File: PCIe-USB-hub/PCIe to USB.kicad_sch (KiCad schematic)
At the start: 105 parts, among them Y1 X322524MQB4SI, Y2 X322524MQB4SI, Y3 X322524MQB4SI

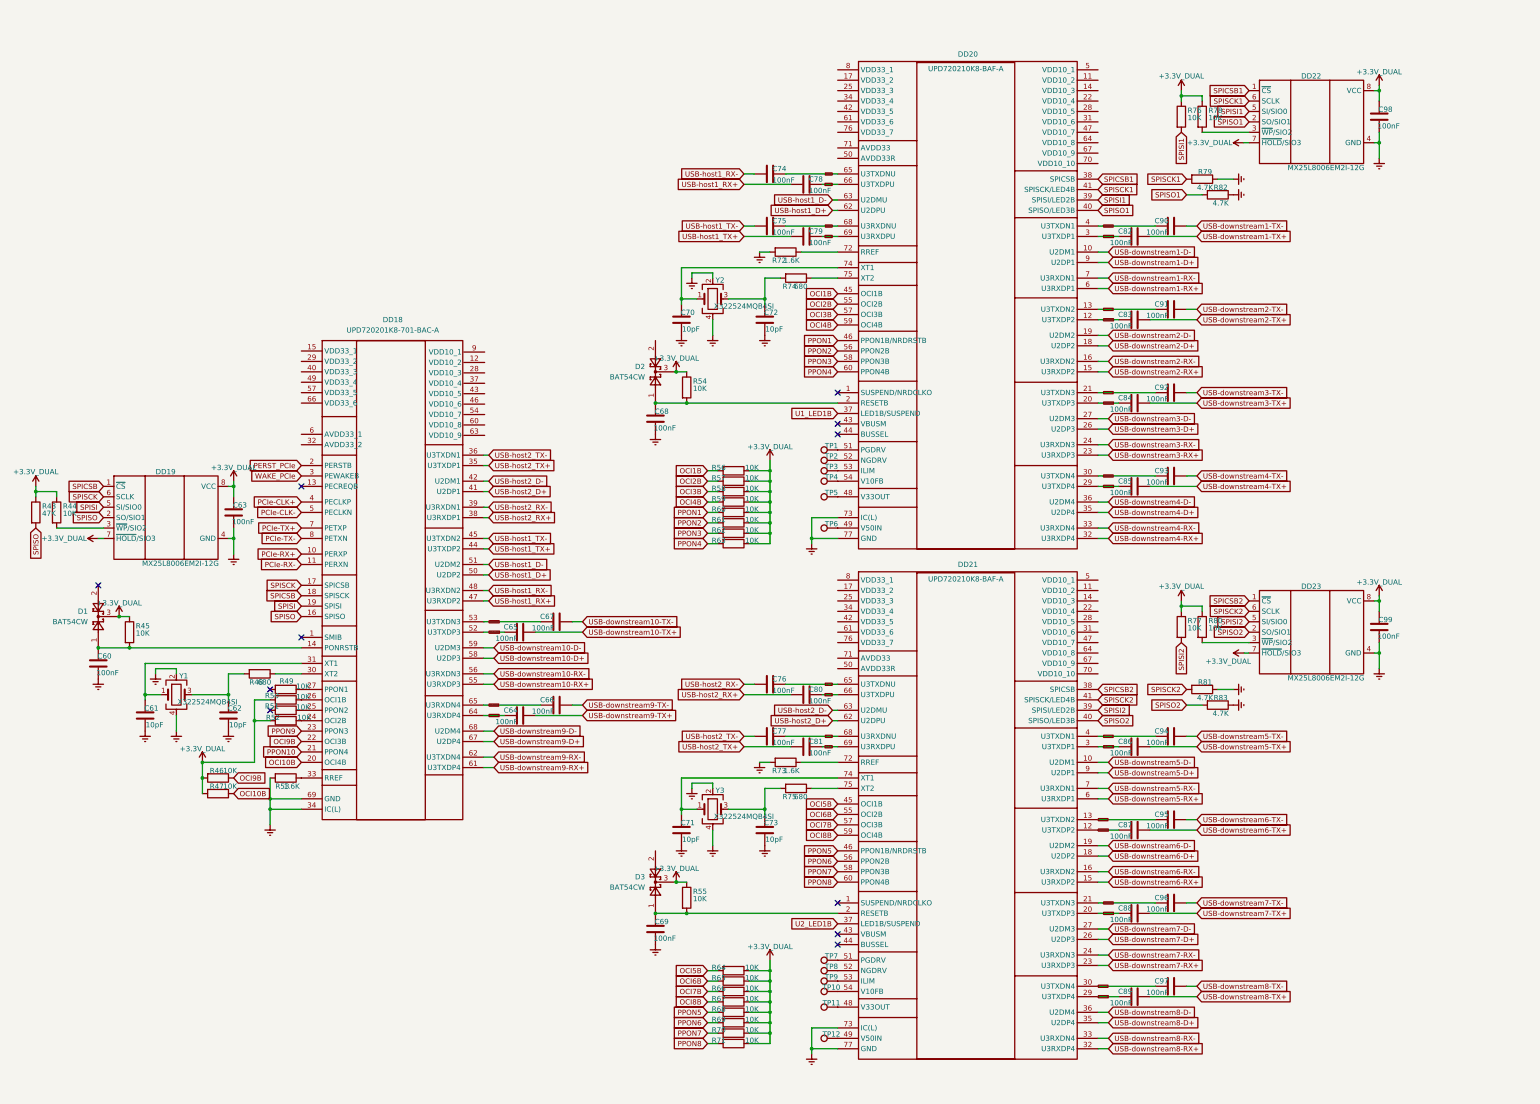
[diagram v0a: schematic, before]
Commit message: тык-перетык
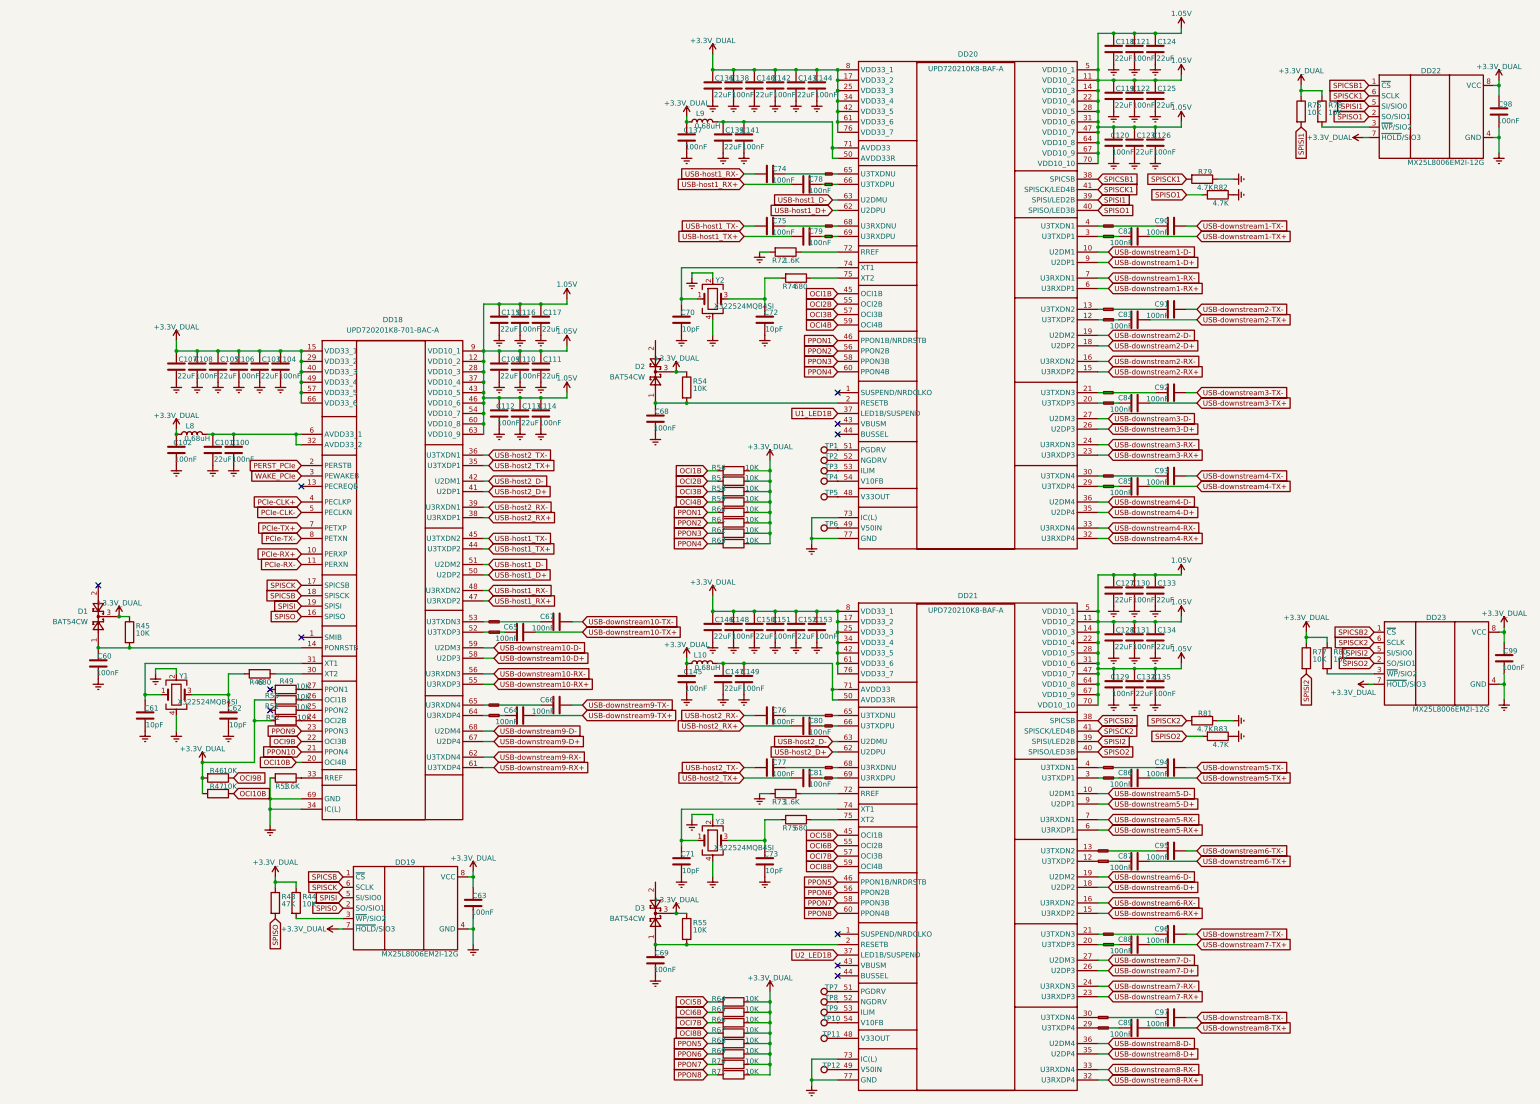
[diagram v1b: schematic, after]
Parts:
- added C100, C102, C104, C106, C108, C110, C112, C114, C116, C120, C121, C122, C126, C129, C130, C131, C135, C137, C138, C141, C142, C144, C145, C148, C149, C151, C153: 100nF, Capacitor_SMD:C_0402_1005Metric, symbol Device:C
- added C101, C103, C105, C107, C109, C111, C113, C115, C117, C118, C119, C123, C124, C125, C127, C128, C132, C133, C134, C136, C139, C140, C143, C146, C147, C150, C152: 22uF, Capacitor_SMD:C_0402_1005Metric, symbol Device:C
- added L10, L8, L9: 0.68uH, Inductor_SMD:L_Cenker_CKCS4020, symbol Device:L
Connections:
- net +3.3V_DUAL: now also DD18.15 (VDD33_1), DD18.29 (VDD33_2), DD18.40 (VDD33_3), DD18.49 (VDD33_4), DD18.57 (VDD33_5), DD18.66 (VDD33_6), DD20.17 (VDD33_2), DD20.25 (VDD33_3), DD20.34 (VDD33_4), DD20.42 (VDD33_5), DD20.61 (VDD33_6), DD20.76 (VDD33_7), DD20.8 (VDD33_1), DD21.17 (VDD33_2), DD21.25 (VDD33_3), DD21.34 (VDD33_4), DD21.42 (VDD33_5), DD21.61 (VDD33_6), DD21.76 (VDD33_7), DD21.8 (VDD33_1), C102.1, C103.1, C104.1, C105.1, C106.1, C107.1, C108.1, C136.1, C137.1, C138.1, C140.1, C142.1, C143.1, C144.1, C145.1, C146.1, C148.1, C150.1, C151.1, C152.1, C153.1, L10.1, L8.1, L9.1
- net Earth: now also C100.2, C101.2, C102.2, C103.2, C104.2, C105.2, C106.2, C107.2, C108.2, C109.2, C110.2, C111.2, C112.2, C113.2, C114.2, C115.2, C116.2, C117.2, C118.2, C119.2, C120.2, C121.2, C122.2, C123.2, C124.2, C125.2, C126.2, C127.2, C128.2, C129.2, C130.2, C131.2, C132.2, C133.2, C134.2, C135.2, C136.2, C137.2, C138.2, C139.2, C140.2, C141.2, C142.2, C143.2, C144.2, C145.2, C146.2, C147.2, C148.2, C149.2, C150.2, C151.2, C152.2, C153.2
- net 1.05V: now reaches DD18.12 (VDD10_2)
- net 1.05V: now also DD18.28 (VDD10_3), DD18.37 (VDD10_4), DD18.43 (VDD10_5), DD18.46 (VDD10_6), DD18.54 (VDD10_7), DD18.60 (VDD10_8), DD18.63 (VDD10_9), DD18.9 (VDD10_1), DD20.11 (VDD10_2), DD20.14 (VDD10_3), DD20.22 (VDD10_4), DD20.28 (VDD10_5), DD20.31 (VDD10_6), DD20.47 (VDD10_7), DD20.5 (VDD10_1), DD20.64 (VDD10_8), DD20.67 (VDD10_9), DD20.70 (VDD10_10), DD21.11 (VDD10_2), DD21.14 (VDD10_3), DD21.22 (VDD10_4), DD21.28 (VDD10_5), DD21.31 (VDD10_6), DD21.47 (VDD10_7), DD21.5 (VDD10_1), DD21.64 (VDD10_8), DD21.67 (VDD10_9), DD21.70 (VDD10_10), C109.1, C110.1, C111.1, C112.1, C113.1, C114.1, C115.1, C116.1, C117.1, C118.1, C119.1, C120.1, C121.1, C122.1, C123.1, C124.1, C125.1, C126.1, C127.1, C128.1, C129.1, C130.1, C131.1, C132.1, C133.1, C134.1, C135.1
- net at DD18.32 (AVDD33_2): now also DD18.6 (AVDD33_1), C100.1, C101.1, L8.2
- net at DD20.50 (AVDD33R): now also DD20.71 (AVDD33), C139.1, C141.1, L9.2
- net at DD21.50 (AVDD33R): now also DD21.71 (AVDD33), C147.1, C149.1, L10.2
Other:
- moved on the sheet: C63, C69, C71, C73, C76, C77, C80, C81, C86, C87, C88, C89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
